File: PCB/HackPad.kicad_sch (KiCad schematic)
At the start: 22 parts, among them SW1 SW_Push, SW2 SW_Push, SW3 SW_Push, SW4 SW_Push, SW5 SW_Push, SW6 SW_Push, SW7 SW_Push, SW8 SW_Push, SW9 SW_Push, U1 XIAO-RP2040-DIP, U2 SSD1306

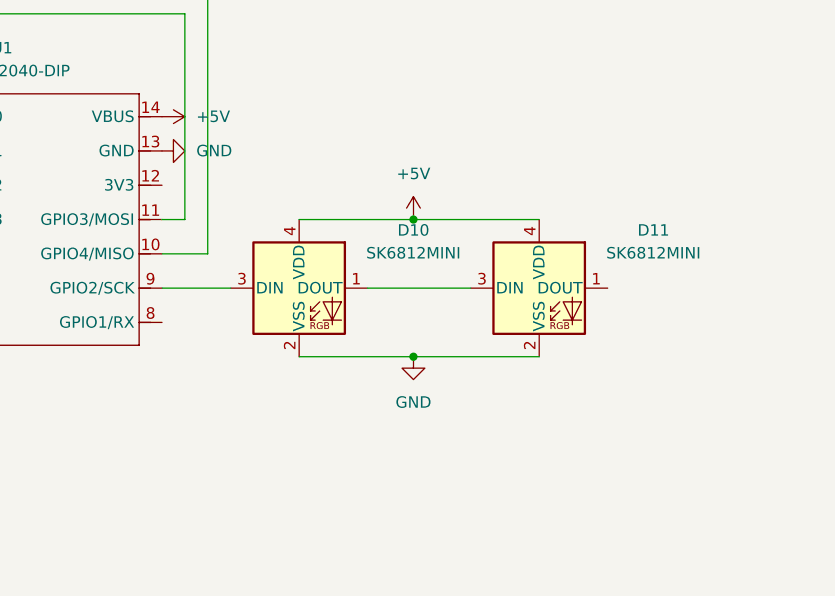
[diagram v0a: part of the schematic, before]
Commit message: Add files via upload
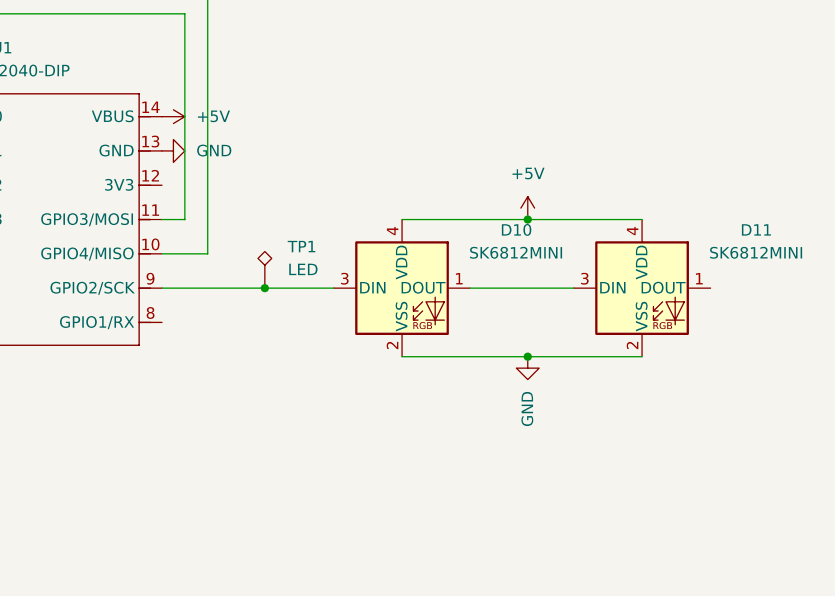
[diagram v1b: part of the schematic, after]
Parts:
- added TP1: LED, TestPoint:TestPoint_Pad_D2.0mm, symbol Connector:TestPoint_Alt
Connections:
- net at D10.3 (DIN), U1.9 (GPIO2/SCK): now also TP1.1
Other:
- moved on the sheet: D10, D11
